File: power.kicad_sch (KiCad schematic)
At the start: 24 parts

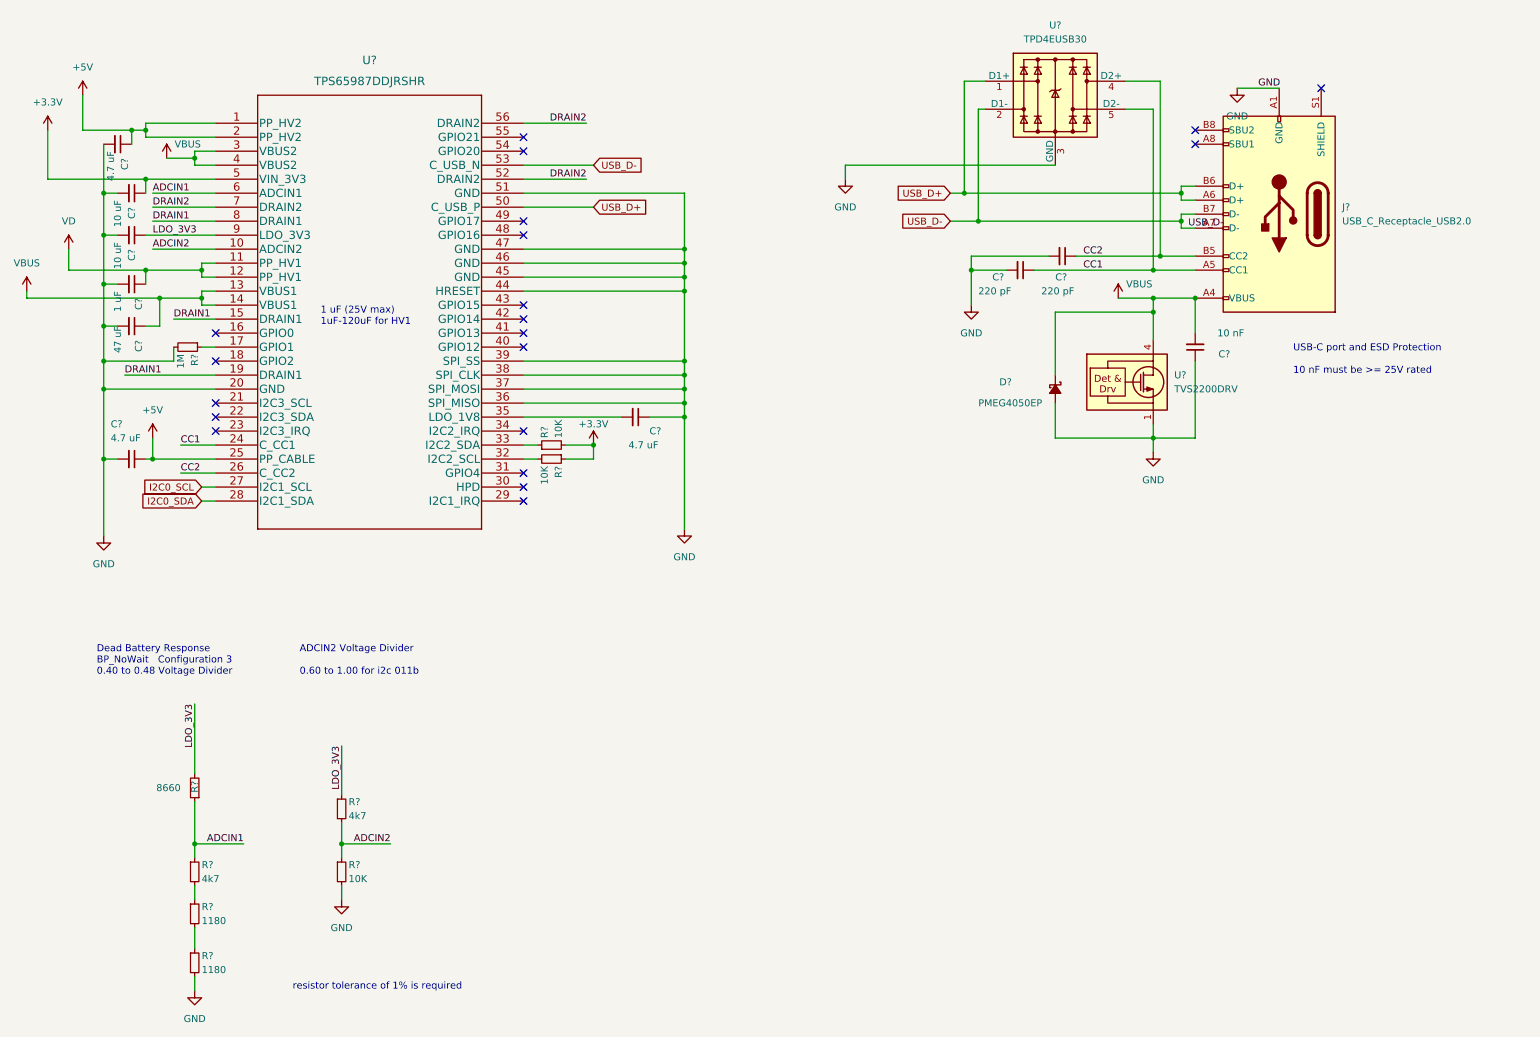
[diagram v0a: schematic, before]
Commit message: production version (2023)
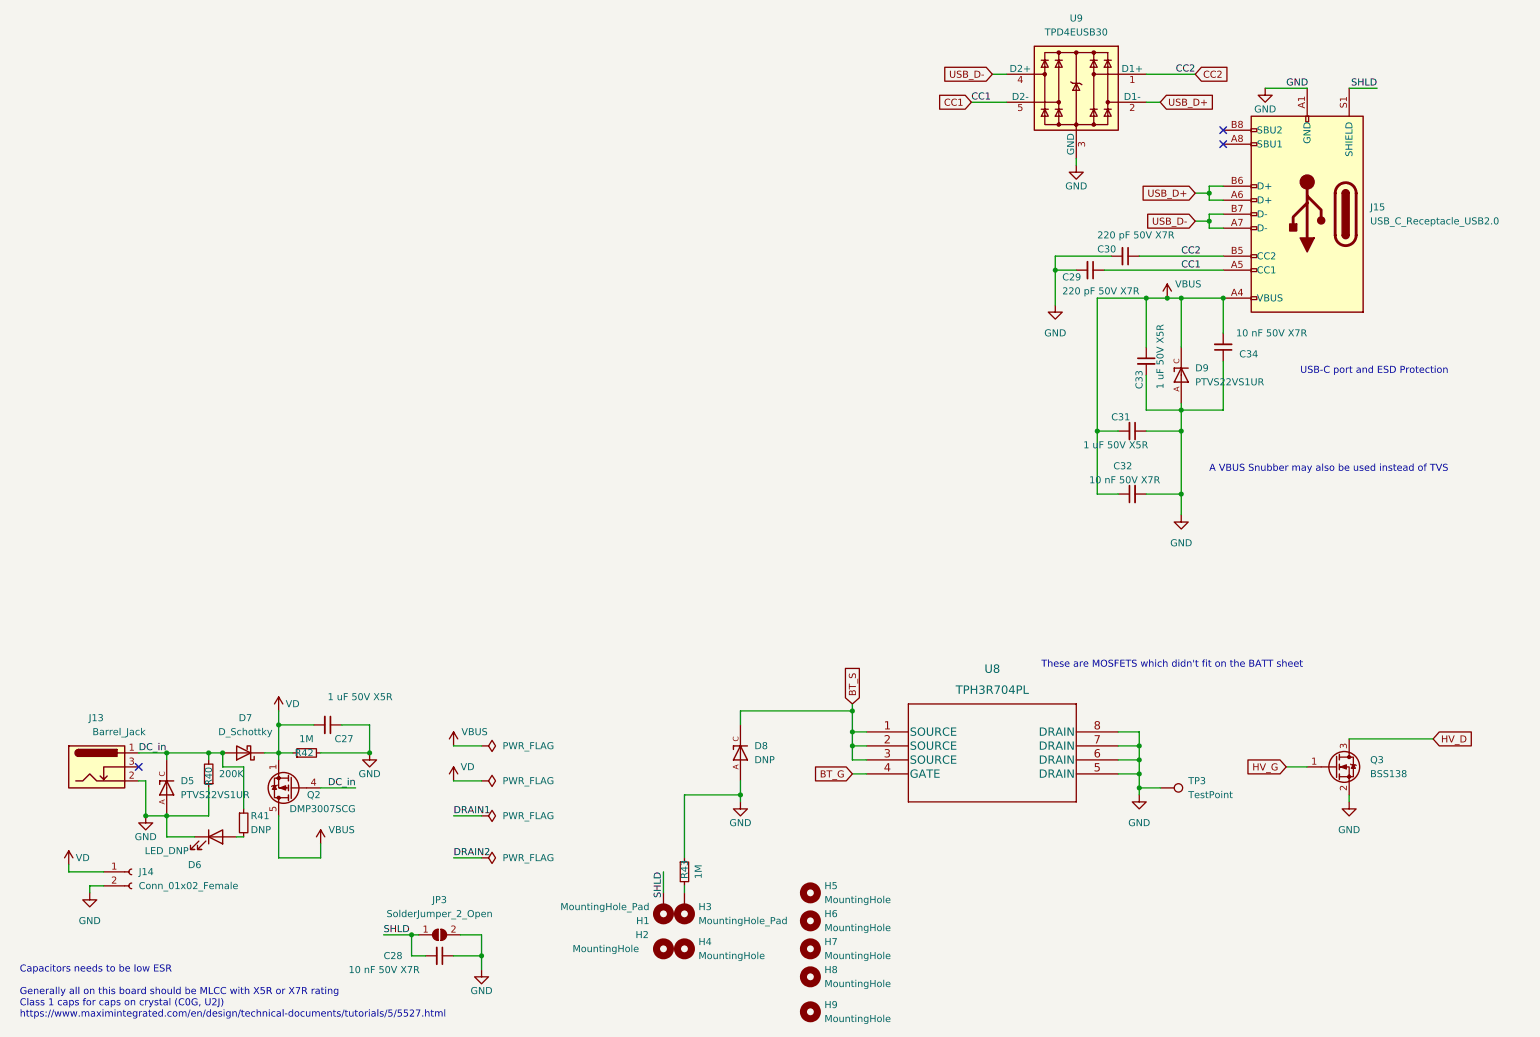
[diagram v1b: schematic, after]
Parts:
- removed C? (x3): 4.7 uF, symbol Device:C_Small
- removed C? (x2): 10 uF, symbol Device:C_Small
- removed C?: 1 uF, symbol Device:C_Small
- removed D?: PMEG4050EP, symbol Device:D_Schottky_Small_Filled
- removed R? (x2): 4k7, symbol Device:R_Small
- removed R? (x2): 1180, symbol Device:R_Small
- removed R? (x3): 10K, symbol Device:R_Small
- removed R?: 1M, symbol Device:R_Small
- removed R?: 8660, symbol Device:R_Small
- removed U?: TVS2200DRV, Package_SON:WSON-6-1EP_2x2mm_P0.65mm_EP1x1.6mm, symbol Power_Protection:TVS2200DRV
- removed U?: TPS65987DDJRSHR, PowerIC:TPS65987DDJRSHR, symbol TPS65987DDJRSHR:TPS65987DDJRSHR
- added C27, C31: 1 uF 50V X5R, Capacitor_SMD:C_0603_1608Metric, symbol Device:C_Small
- added C28, C32: 10 nF 50V X7R, Capacitor_SMD:C_0402_1005Metric_Pad0.74x0.62mm_HandSolder, symbol Device:C_Small
- added D5, D9: PTVS22VS1UR, PowerIC:TVS_PTVS22VS1UR, symbol PTVS22VS1UR:PTVS22VS1UR
- added D6: LED_DNP, LED_SMD:LED_0805_2012Metric_Pad1.15x1.40mm_HandSolder, symbol Device:LED
- added D7: D_Schottky, Diode_SMD:D_SMA, symbol Device:D_Schottky
- added D8: DNP, PowerIC:TVS_PTVS22VS1UR, symbol PTVS22VS1UR:PTVS22VS1UR
- added H1, H3: MountingHole_Pad, MountingHole:MountingHole_3.2mm_M3_Pad, symbol Mechanical:MountingHole_Pad
- added H2: MountingHole, MountingHole:MountingHole_3.2mm_M3, symbol Mechanical:MountingHole
- added H4: MountingHole, MountingHole:MountingHole_3.2mm_M3_ISO7380, symbol Mechanical:MountingHole
- added H5: MountingHole, MountingHole:MountingHole_8.4mm_M8, symbol Mechanical:MountingHole
- added H6, H7, H8, H9: MountingHole, MountingHole:MountingHole_2.7mm_M2.5, symbol Mechanical:MountingHole
- added J13: Barrel_Jack, Connector_BarrelJack:BarrelJack_GCT_DCJ200-10-A_Horizontal, symbol Connector:Barrel_Jack_Switch
- added J14: Conn_01x02_Female, Connector_PinHeader_2.54mm:PinHeader_1x02_P2.54mm_Vertical, symbol Connector:Conn_01x02_Female
- added JP3: SolderJumper_2_Open, Resistor_SMD:R_0805_2012Metric_Pad1.20x1.40mm_HandSolder, symbol Jumper:SolderJumper_2_Open
- added Q2: DMP3007SCG, Package_SON:Diodes_PowerDI3333-8, symbol Transistor_FET:DMP3013SFV
- added Q3: BSS138, Package_TO_SOT_SMD:SOT-23, symbol Transistor_FET:AO3400A
- added R40: 200K, Capacitor_SMD:C_0402_1005Metric_Pad0.74x0.62mm_HandSolder, symbol Device:R_Small
- added R41: DNP, Resistor_SMD:R_0805_2012Metric_Pad1.20x1.40mm_HandSolder, symbol Device:R_Small
- added R42, R43: 1M, Capacitor_SMD:C_0402_1005Metric_Pad0.74x0.62mm_HandSolder, symbol Device:R_Small
- added TP3: TestPoint, TestPoint:TestPoint_Pad_4.0x4.0mm, symbol Connector:TestPoint
- added U8: TPH3R704PL, PowerIC:TRANS_TPHR8504PL,L1Q, symbol TPN5R203PL:TPN5R203PL
- C29, C30: renamed from C?; value 220 pF -> 220 pF 50V X7R; footprint (none) -> Capacitor_SMD:C_0402_1005Metric_Pad0.74x0.62mm_HandSolder; JCLPCB (none) -> C1530; Vendor (none) -> C1530
- C33: renamed from C?; value 47 uF -> 1 uF 50V X5R; footprint (none) -> Capacitor_SMD:C_0603_1608Metric; JCLPCB (none) -> C15849; Vendor (none) -> C15849
- C34: renamed from C?; value 10 nF -> 10 nF 50V X7R; footprint (none) -> Capacitor_SMD:C_0402_1005Metric_Pad0.74x0.62mm_HandSolder; JCLPCB (none) -> C15195; Vendor (none) -> C15195
- J15: renamed from J?; footprint Connector_USB:USB_C_Receptacle_GCT_USB4085 -> Connector_USB:USB_C_Receptacle_HRO_TYPE-C-31-M-12; JCLPCB (none) -> C165948; Vendor (none) -> C165948
- U9: renamed from U?; JCLPCB (none) -> C558427; Vendor (none) -> C558427
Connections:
- net CC2: now also U9.1 (D1+); no longer U9.4 (D2+)
- net GND: now also C27.1, C28.1, C31.1, C32.2, D5.A, D6.1 (K), D8.A, D9.A, J13.2, J14.2 (Pin_2), JP3.2 (B), Q3.2 (S), R40.1, R42.2, R43.1, TP3.1, U8.5 (DRAIN), U8.6 (DRAIN), U8.7 (DRAIN), U8.8 (DRAIN)
- net USB_D+: now also U9.2 (D1-); no longer U9.1 (D1+)
- net USB_D-: now also U9.4 (D2+); no longer U9.2 (D1-)
- net VBUS: now also C31.2, C32.1, D9.C, Q2.5 (D)
- net VD: now also C27.2, D7.1 (K), J14.1 (Pin_1), Q2.1 (S), Q2.2 (S), Q2.3 (S), R42.1
- net SHLD: now reaches J15.S1 (SHIELD)
- net SHLD: now also C28.2, H1.1, JP3.1 (A)
- new net: D6.2 (A), R41.2
- new net: H3.1, R43.2
- new net BT_G: U8.4 (GATE)
- new net BT_S: D8.C, U8.1 (SOURCE), U8.2 (SOURCE), U8.3 (SOURCE)
- new net DC_in: D5.C, D7.2 (A), J13.1, Q2.4 (G), R40.2, R41.1
- new net HV_D: Q3.3 (D)
- new net HV_G: Q3.1 (G)
- no-connect marks 20 -> 3
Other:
- note added: "A VBUS Snubber may also be used instead of TVS"
- note added: "Capacitors needs to be low ESR Generally all on this board should be MLCC with X5R or X7R rating Class 1 caps for caps on crystal (C0G, U2J) https://www.maximintegrated.com/en/design/technical-documents/tutorials/5/5527.html"
- note added: "These are MOSFETS which didn't fit on the BATT sheet"
- note added: "USB-C port and ESD Protection"
- note removed: "1 uF (25V max) 1uF-120uF for HV1"
- note removed: "ADCIN2 Voltage Divider 0.60 to 1.00 for i2c 011b"
- note removed: "Dead Battery Response BP_NoWait Configuration 3 0.40 to 0.48 Voltage Divider"
- note removed: "USB-C port and ESD Protection 10 nF must be >= 25V rated"
- note removed: "resistor tolerance of 1% is required"
- moved on the sheet: C29, C30, C33, C34, J15, U9
